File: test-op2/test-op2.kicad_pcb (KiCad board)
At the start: 2 copper layers, 167 parts, among them P1 In1, P10 Out2, P11 Out3, P12 Out4, P13 CONN_13X2, P14 CONN_5X2, P2 In2, P3 In3, P4 In4, P5 HOLD3, P6 RST3, P7 HOLD4, P8 RST4, P9 Out1, U1 LM7171, U10 LM7171, U11 LMH6505, U12 LMH6505, U13 DG467, U14 DG468, U15 LM7171, U16 LMH6505, U17 LMH6505, U2 LMH6505, U3 LMH6505, U4 LM7171, U5 LMH6505, U6 LMH6505, U7 DG467, U8 DG468, U9 LM7171

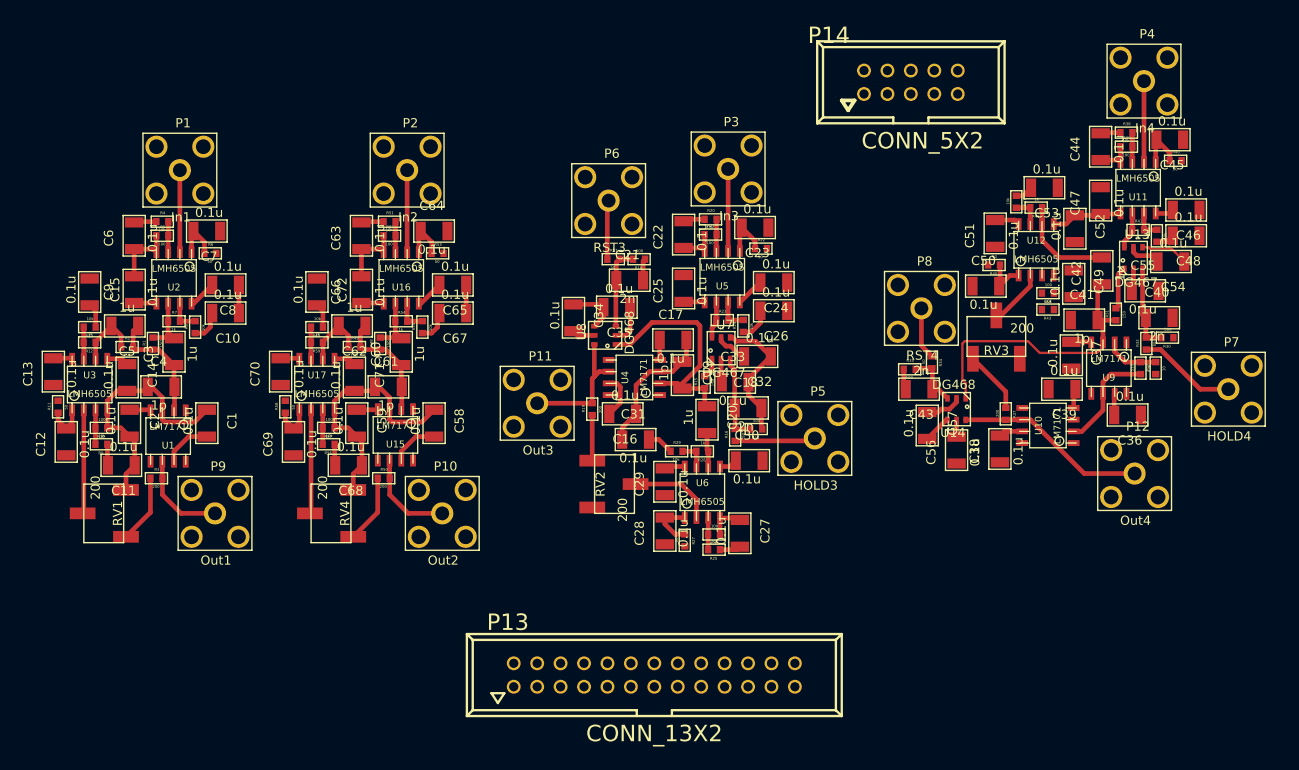
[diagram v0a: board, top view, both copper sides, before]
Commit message: [test-op2] layout
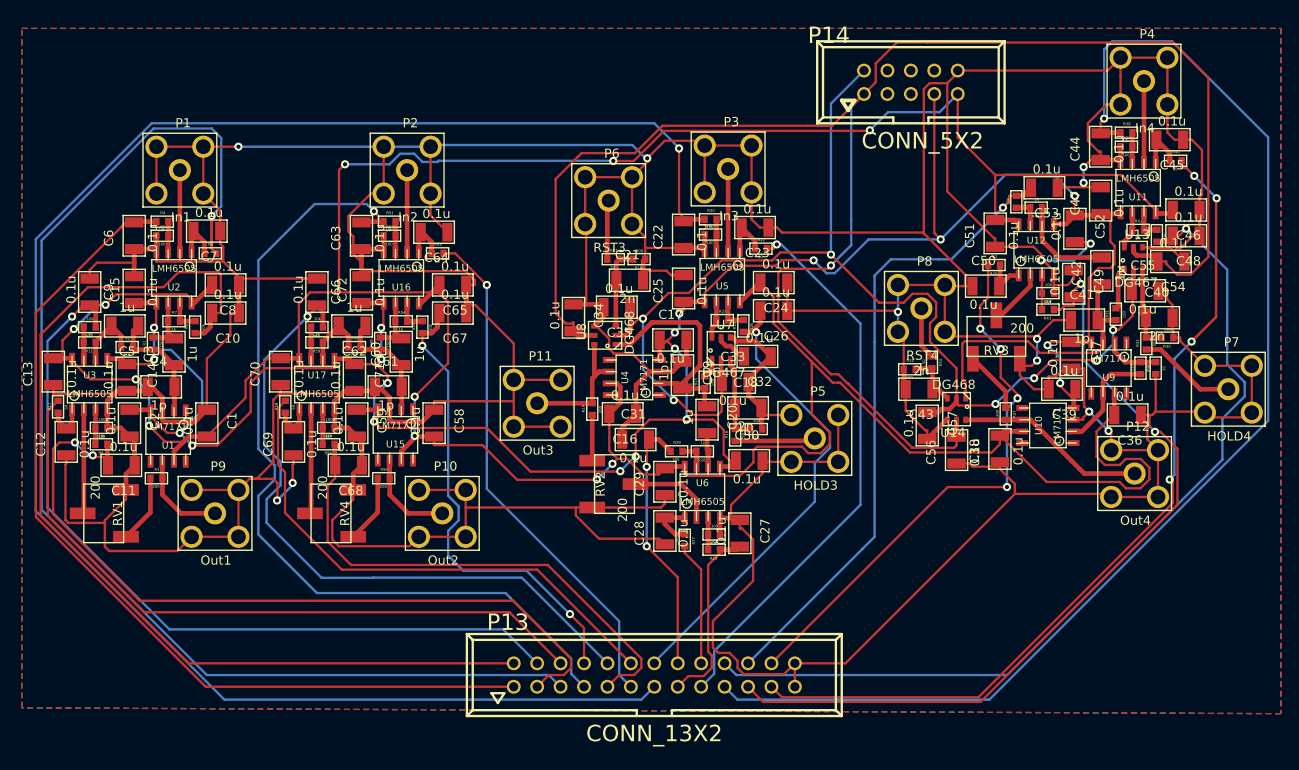
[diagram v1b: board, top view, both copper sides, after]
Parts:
- moved C64 0.13 mm to (148.2, 39.2), turned to 0 degrees
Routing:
- net GND: track 137.5 -> 957.2 mm, vias 0 -> 13
- net +5V: track 40.8 -> 382.2 mm, vias 0 -> 11
- net -5V: track 32.8 -> 258.6 mm, vias 0 -> 19
- net Off1_3: track 2.35 -> 192.0 mm, vias 0 -> 1
- net +15V: track 11.4 -> 193.0 mm, vias 0 -> 1
- net Ctrl1_1: track 0.00 -> 135.0 mm, vias 0 -> 1
- net Off1_4: track 2.17 -> 136.6 mm, vias 0 -> 1
- net -15V: track 13.4 -> 132.7 mm, vias 0 -> 7
- net Off2_1: track 3.53 -> 108.6 mm
- net Ctrl1_4: track 0.00 -> 97.7 mm, vias 0 -> 4
- net Off1_1: track 2.43 -> 98.7 mm
- net Off2_4: track 1.99 -> 96.6 mm, vias 0 -> 1
- net Off1_2: track 2.43 -> 93.4 mm, vias 0 -> 1
- net Off3_4: track 0.00 -> 89.8 mm, vias 0 -> 2
- net Off4_1: track 2.63 -> 86.9 mm, vias 0 -> 1
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- added copper zone on B.Cu, net GND
- added copper zone on F.Cu, net GND
